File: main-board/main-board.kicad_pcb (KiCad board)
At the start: 2 copper layers, 69 parts, among them J1 NVIDIA_Jetson_NX_Dev_40pin_Co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, J10 FSESC_6.6_COMM_Minimal, J11 FSESC_6.6_COMM_Minimal, J12 FSESC_6.6_COMM_Minimal, J13 FSESC_6.6_COMM_Minimal, J14 ArducamPTZ, J2 NVIDIA_Jetson_NX_Dev_Button_C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, J3 Conn_01x02, J4 Conn_01x02, J5 Conn_01x02, J6 FSESC_6.6_COMM_Minimal, J7 QWIIC_Generic_Conn, J8 Conn_01x03, J9 FSESC_6.6_COMM_Minimal, M1 Fan_3pin, M2 Fan_3pin, M3 Fan_3pin, Q1 Q_NMOS_GSD, Q2 Q_NMOS_GSD, Q4 Q_NMOS_GSD, Q5 Q_NMOS_GSD, Q6 Q_NMOS_GSD, Q7 Q_NMOS_GSD, Q8 Q_NMOS_GSD, U1 RFM95W_Adafruit_Breakout, U10 Analog Temp Sensor, U11 Adafruit_GPS_V3, U12 SN74AHCT125D, U2 TDK_I3A4W008A033V, U3 TDK_I3A4W008A033V, U5 Teensy_4.1, U6 Analog Temp Sensor, U7 Analog Temp Sensor, U8 Analog Temp Sensor, U9 Analog Temp Sensor

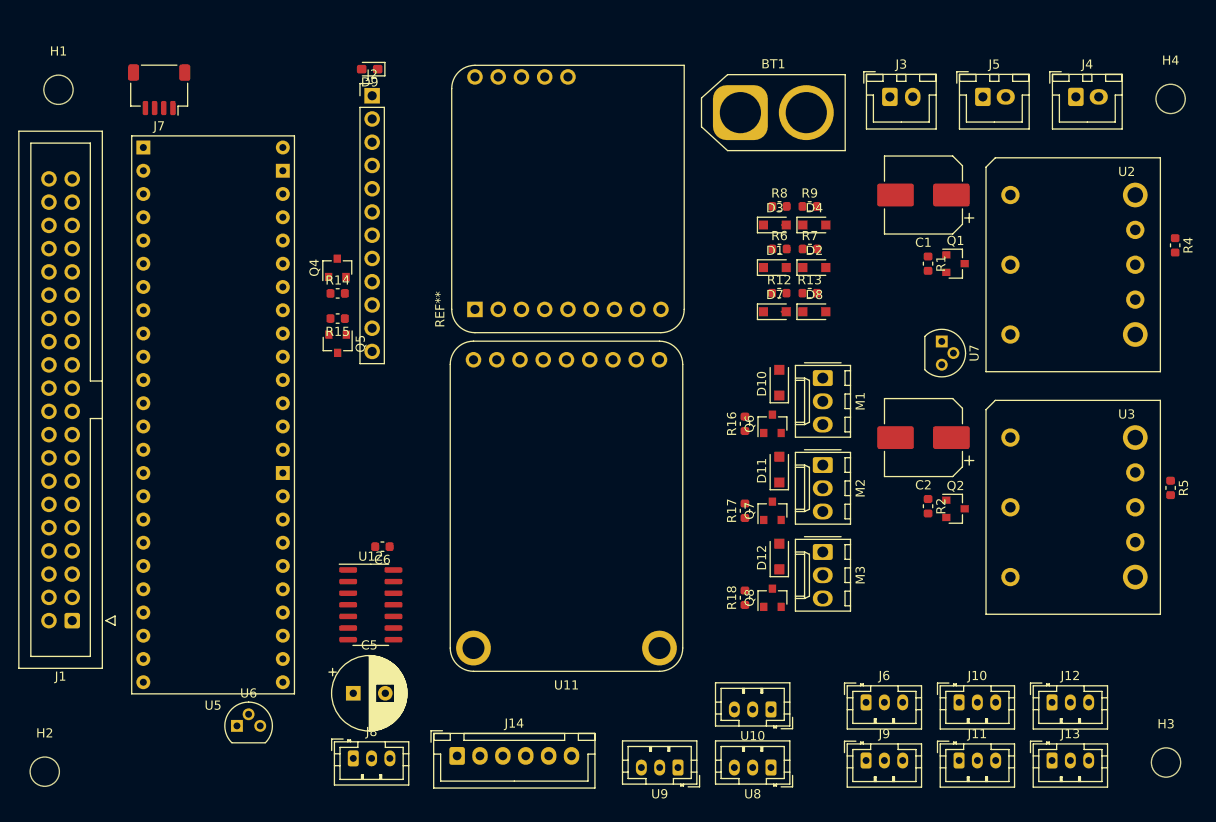
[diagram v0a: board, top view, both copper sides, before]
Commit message: Started routing
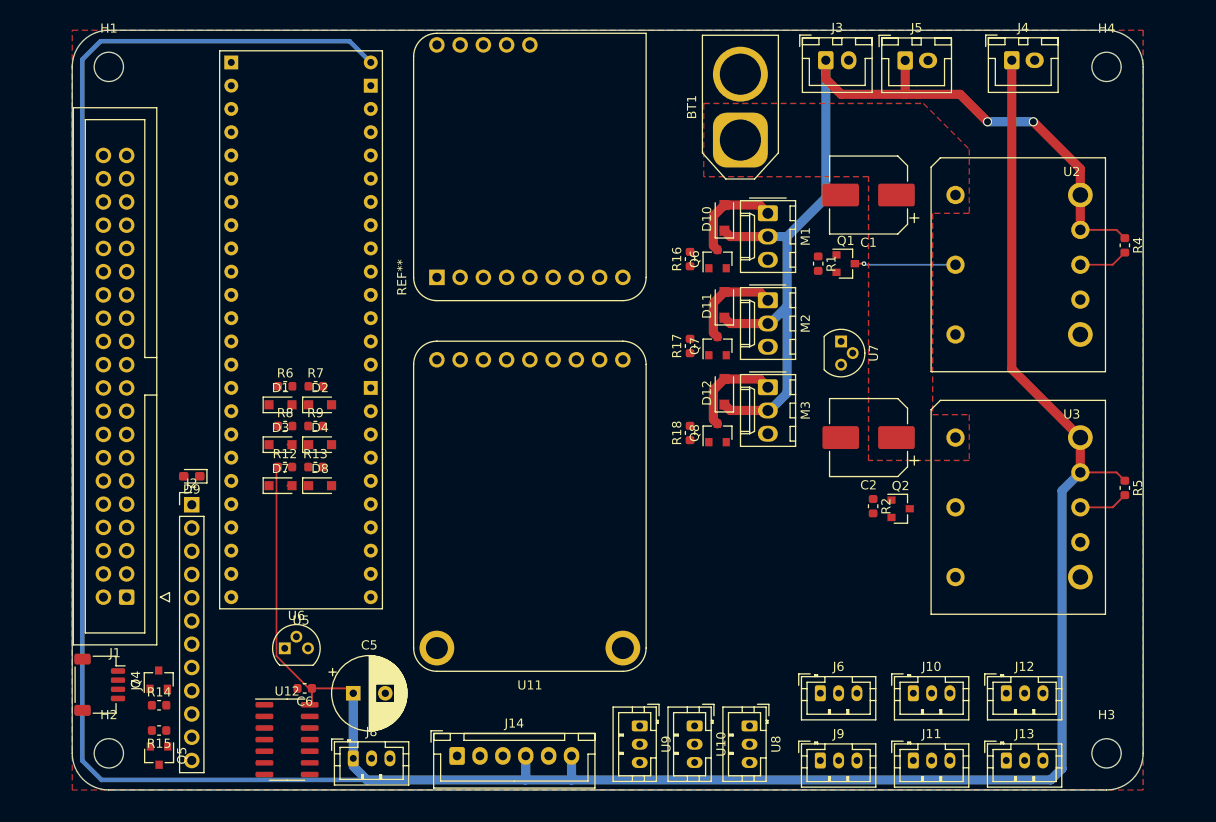
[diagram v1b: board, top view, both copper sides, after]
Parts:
- moved J7 65.3 mm to (99.0, 132.5), turned to 270 degrees
- moved D4 59.1 mm to (123.1, 106.3)
- moved R8 59.1 mm to (119.3, 104.2)
- moved R9 59.1 mm to (122.6, 104.2)
- moved D3 59.1 mm to (118.8, 106.3)
- moved D8 57.2 mm to (123.1, 110.8)
- moved R12 57.2 mm to (119.2, 108.7)
- moved R13 57.2 mm to (122.6, 108.7)
- moved D7 57.2 mm to (118.8, 110.8)
- moved D2 56.0 mm to (123.1, 101.9)
- moved R6 56.0 mm to (119.3, 99.9)
- moved D1 56.0 mm to (118.8, 101.9)
- moved R7 56.0 mm to (122.6, 99.9)
- moved Q5 49.0 mm to (105.5, 140.2)
- moved R14 49.0 mm to (105.5, 134.8)
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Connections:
- U5 pad 16: /GPS_TX -> GND
- U5 pad 17: /GPS_RX -> /M3_TX
- U5 pad 18: /ADC3 -> /SCK
- U5 pad 19: /ADC4 -> /M3_RX
- U5 pad 20: /M5_RX -> (no net)
- U5 pad 21: /M5_TX -> (no net)
- U5 pad 22: /12V_Disable -> /ADC1
- U5 pad 23: /5V_Disable -> /ADC2
- U5 pad 24: (no net) -> /M4_TX
- U5 pad 25: /Fan1_Control -> /M4_RX
- U5 pad 26: /M6_RX -> (no net)
- U5 pad 27: /M6_TX -> (no net)
- U5 pad 28: /Fan2_Control -> +3V3
- U5 pad 29: /Fan3_Control -> GND
- U5 pad 30: /ADC_5V -> +5V
- U5 pad 31: /ADC_12V -> /GPS_TX
- U5 pad 32: /ADC_BATT -> /GPS_RX
- U5 pad 33: /ADC5 -> /ADC3
- U5 pad 34: GND -> /ADC4
- U5 pad 35: /SCK -> /M5_RX
- U5 pad 36: /M3_TX -> /M5_TX
- U5 pad 37: /M3_RX -> /12V_Disable
- U5 pad 38: (no net) -> /5V_Disable
- U5 pad 40: /ADC1 -> /Fan1_Control
- U5 pad 41: /ADC2 -> /M6_RX
- U5 pad 42: /M4_TX -> /M6_TX
- U5 pad 43: /M4_RX -> /Fan2_Control
- U5 pad 44: (no net) -> /Fan3_Control
- U5 pad 45: (no net) -> /ADC_5V
- U5 pad 46: +3V3 -> /ADC_12V
- U5 pad 47: GND -> /ADC_BATT
- U5 pad 48: +5V -> /ADC5
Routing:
- net +5V: track 0.00 -> 352.9 mm
- net +12V: track 0.00 -> 110.5 mm, vias 0 -> 2
- net Net-(Q1-Pad3): track 0.00 -> 11.0 mm, vias 0 -> 1
- net Net-(D12-Pad2): track 0.00 -> 10.7 mm
- net Net-(D11-Pad2): track 0.00 -> 10.7 mm
- net Net-(D10-Pad2): track 0.00 -> 10.7 mm
- net Net-(R5-Pad2): track 0.00 -> 5.41 mm
- net Net-(R4-Pad2): track 0.00 -> 5.41 mm
- added copper zone on F.Cu, net +BATT
- added copper zone on F.Cu, net GND
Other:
- board outline added: 117 x 83 mm
- net class Default: clearance 0.2 -> 0.1524; trace_width 0.25 -> 0.1524; via_dia 0.8 -> 0.508; via_drill 0.4 -> 0.254
- rule pad_to_mask_clearance: 0 -> 0.0508
- rule trace_clearance: 0.2 -> 0.1524
- rule trace_min: 0.2 -> 0.1524
- rule via_min_drill: 0.3 -> 0.254
- rule via_min_size: 0.4 -> 0.508
